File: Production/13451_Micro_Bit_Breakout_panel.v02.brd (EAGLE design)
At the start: 234.2 x 106.4 mm, 108 parts, among them J1 EDGE-80PTH-RA, J10 EDGE-80PTH-RA, J11 M22PTH, J12 EDGE-80PTH-RA, J13 M22PTH, J14 EDGE-80PTH-RA, J15 M22PTH, J16 EDGE-80PTH-RA, J17 M22PTH, J18 EDGE-80PTH-RA, J2 M22PTH, J3 M22PTH, J4 EDGE-80PTH-RA, J5 M22PTH, J6 EDGE-80PTH-RA, J7 M22PTH, J8 EDGE-80PTH-RA, J9 M22PTH

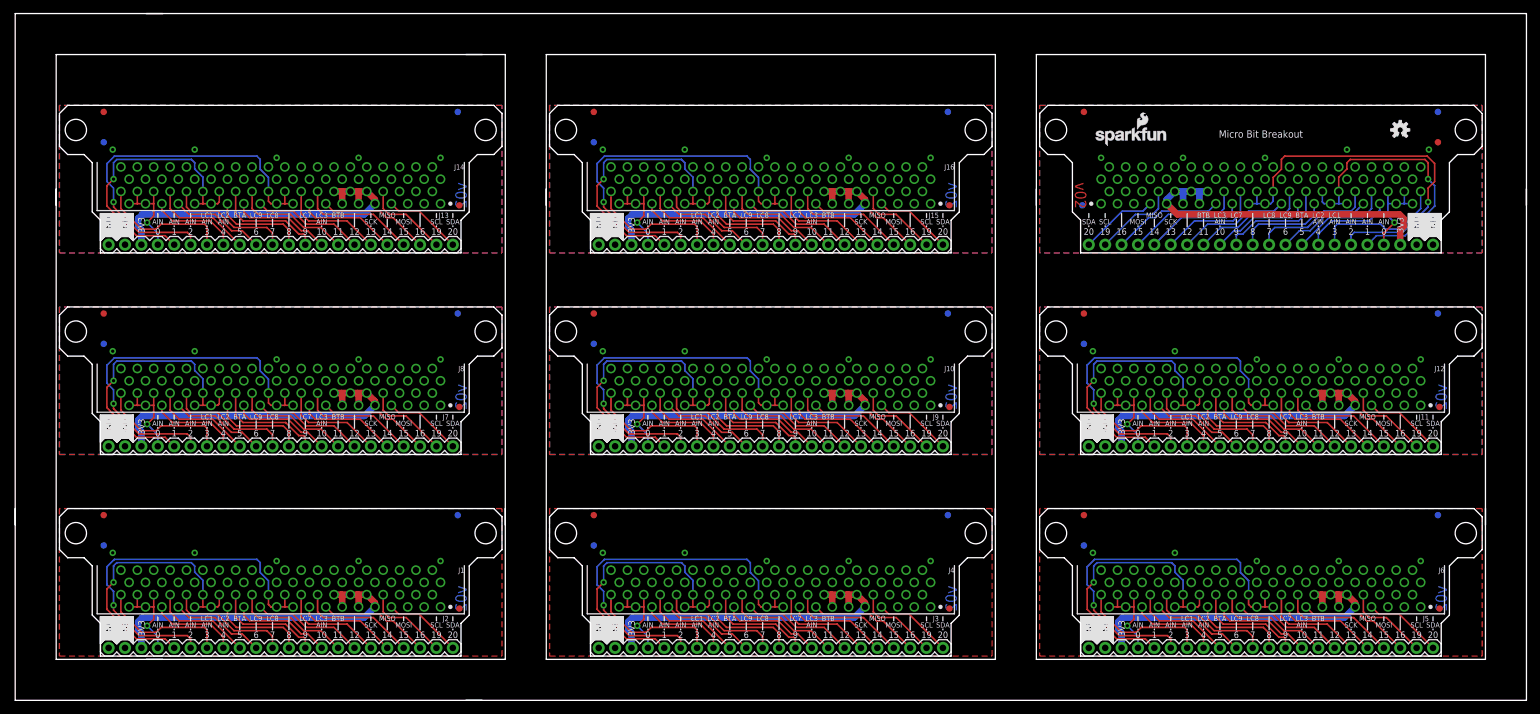
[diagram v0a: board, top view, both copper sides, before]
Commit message: panel
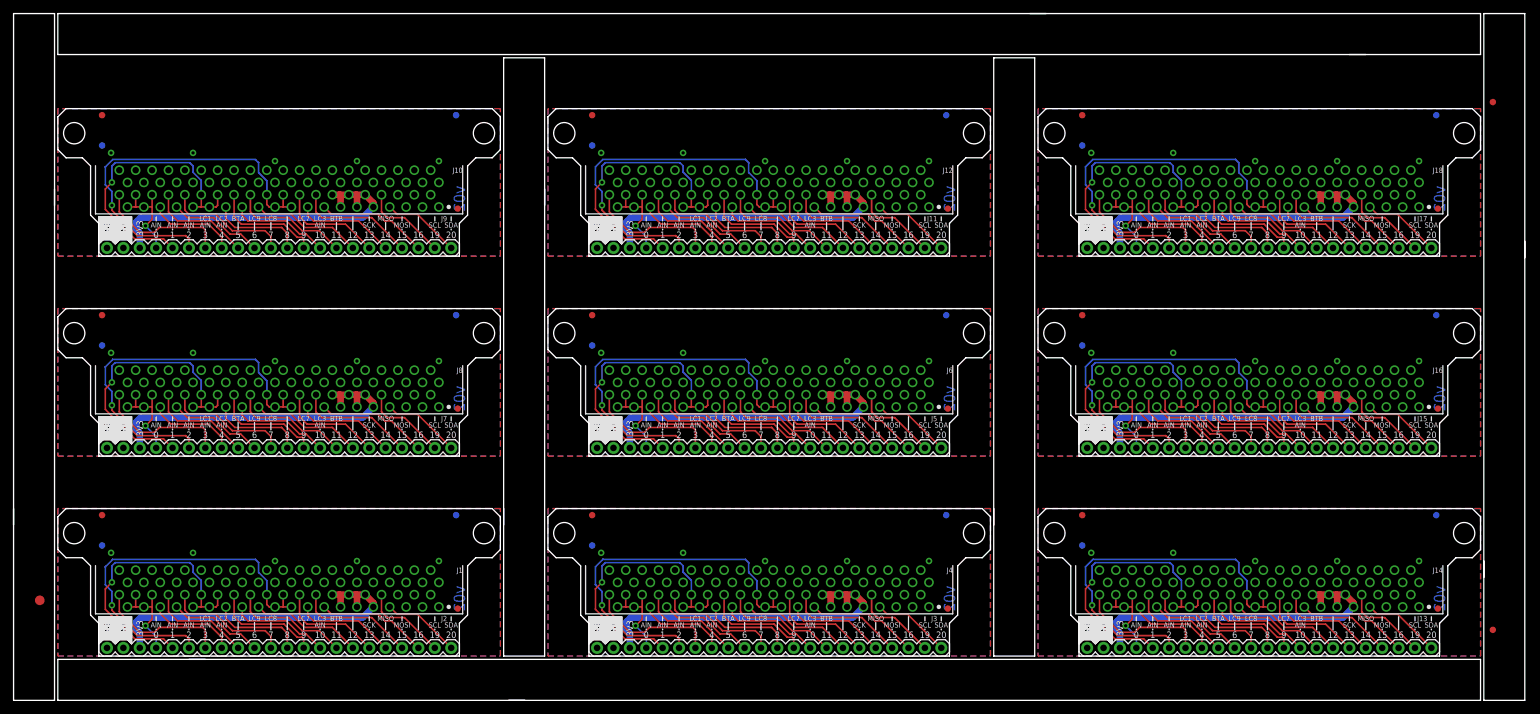
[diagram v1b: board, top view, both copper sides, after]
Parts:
- added E$1: (no value), SparkFun-Retired:FIDUCIAL-1.5X3
- added E$10, E$9: (no value), SparkFun-Aesthetics:FIDUCIAL-1X2
- moved FD25 164.0 mm to (165.6, 28.7)
- moved FD26 164.0 mm to (220.7, 14.2)
- moved FD27 164.0 mm to (220.5, 28.7)
- moved FD28 164.0 mm to (165.6, 24.0)
- moved H13 164.0 mm to (161.3, 25.9)
- moved J13 164.0 mm to (166.4, 8.13)
- moved LOGO14 164.0 mm to (219.1, 23.4)
- moved U$13 164.0 mm to (165.1, 8.76)
- moved U$14 164.0 mm to (170.2, 8.76)
- moved H14 164.0 mm to (224.8, 25.9)
- moved J14 164.0 mm to (193.0, 14.5)
- moved LOGO13 164.0 mm to (171.4, 25.9)
- moved H5 82.3 mm to (85.3, 56.9)
- moved H6 82.3 mm to (148.8, 56.9)
- moved J6 82.3 mm to (117.1, 45.5)
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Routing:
- added copper zone on layer 16, net GND
- added copper zone on layer 16, net GND1
- added copper zone on layer 16, net GND2
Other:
- outline, holes or cut-outs redrawn
